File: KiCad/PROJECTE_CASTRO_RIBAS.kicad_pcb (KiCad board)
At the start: 2 copper layers, 114.1 x 85.8 mm, 64 parts, among them J1 DE9_Pins, J2 DE9_Pins, J3 Conn_01x05, J4 Conn_01x02_Pin, K1 Fujitsu_FTR-LYAA005x, K2 Fujitsu_FTR-LYAA005x, SW3 SW_Push_Dual, SW4 SW_Push, SW5 SW_Push, U1 LM2596S-12, U2 LM1117DT-3.3, U20 PIC24HJ128GP502, U3 SN65HVD230, U4 MAX3232, U6 FDC2214, Y1 Crystal

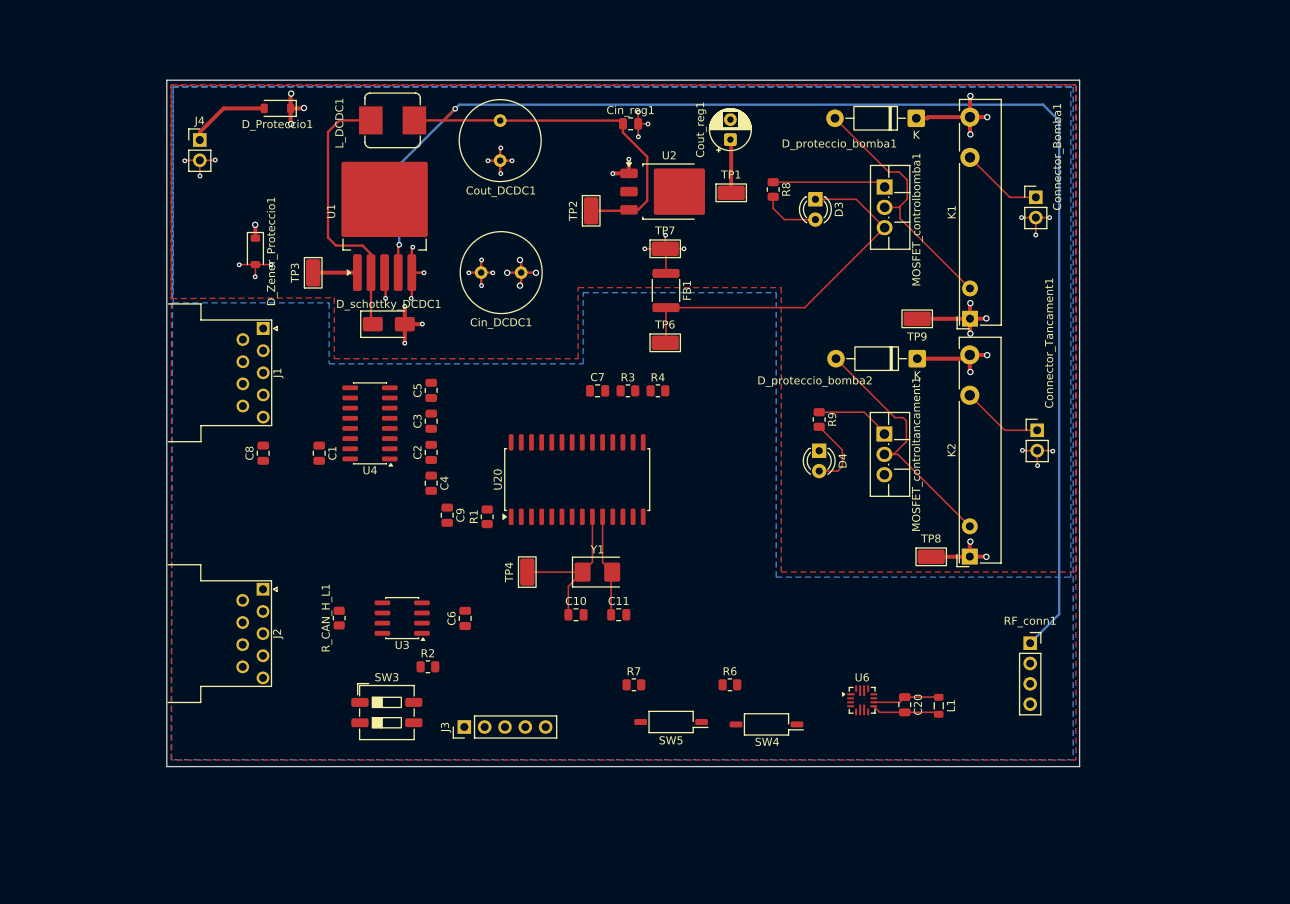
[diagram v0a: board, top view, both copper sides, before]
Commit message: Ruteig V1 fet però falta repassar
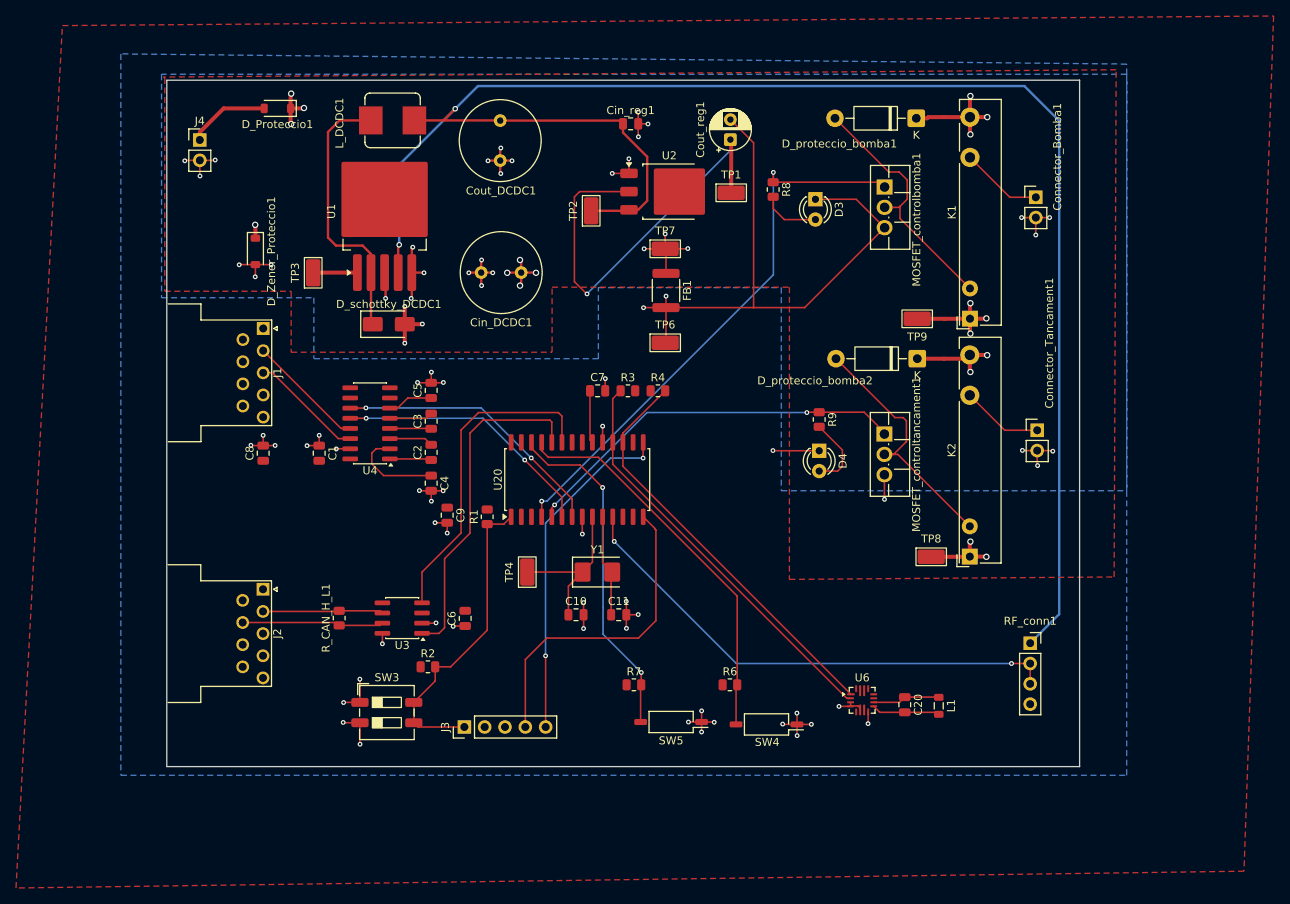
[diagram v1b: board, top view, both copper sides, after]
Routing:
- net GND: track 46.0 -> 150.1 mm, vias 0 -> 43
- net RF_data: track 0.00 -> 64.0 mm, vias 0 -> 2
- net DO_control_bomba: track 14.2 -> 70.8 mm, vias 0 -> 2
- net SCL: track 0.00 -> 51.9 mm
- net SDA: track 0.00 -> 51.4 mm
- net PULS_START: track 0.00 -> 49.1 mm
- net +3.3V: track 6.69 -> 53.3 mm, vias 0 -> 1
- net PGC: track 0.00 -> 43.0 mm, vias 0 -> 2
- net PULS_STOP: track 0.00 -> 43.0 mm, vias 0 -> 2
- net C1TX: track 0.00 -> 42.3 mm
- net C1RX: track 0.00 -> 40.6 mm
- net PGD: track 0.00 -> 40.4 mm
- net MCLR: track 0.00 -> 39.7 mm
- net DO_control_tancament: track 9.41 -> 48.9 mm, vias 0 -> 2
- net TX: track 0.00 -> 34.8 mm, vias 0 -> 2
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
